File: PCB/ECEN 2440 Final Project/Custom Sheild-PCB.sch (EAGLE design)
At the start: 10 parts

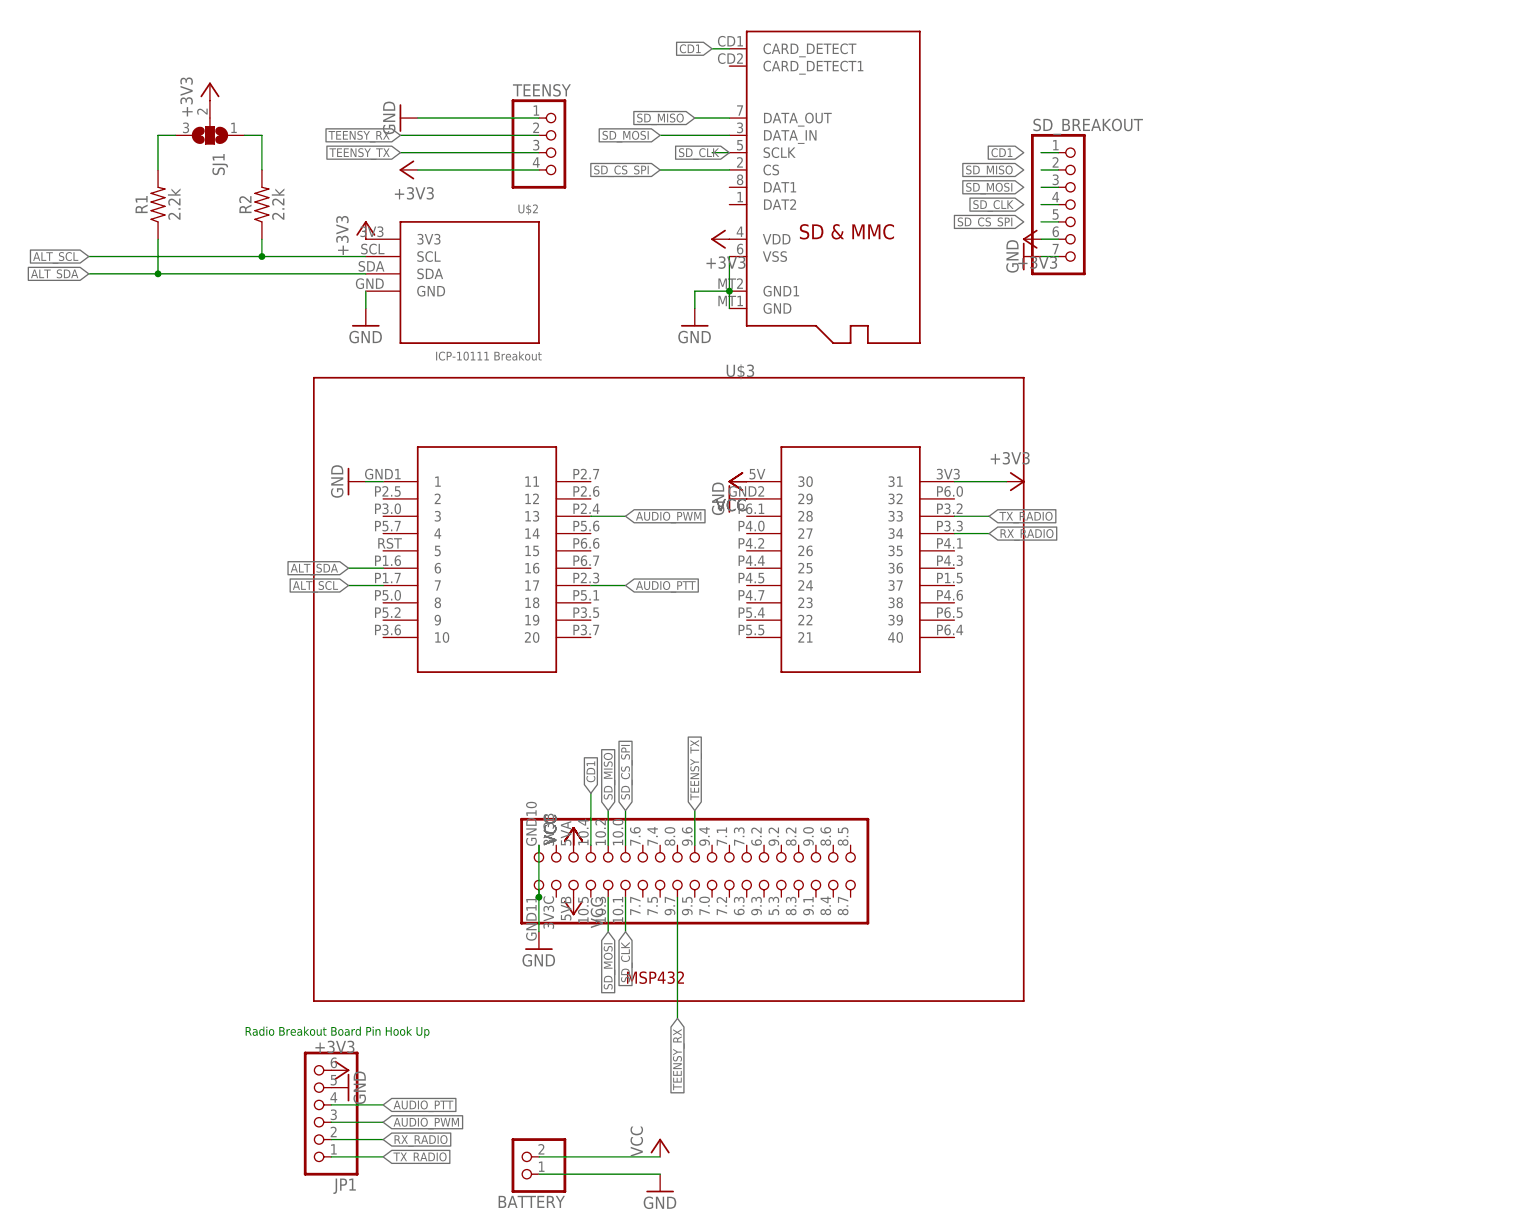
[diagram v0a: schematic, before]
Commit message: prettyfy schematic. vague shield board layout.
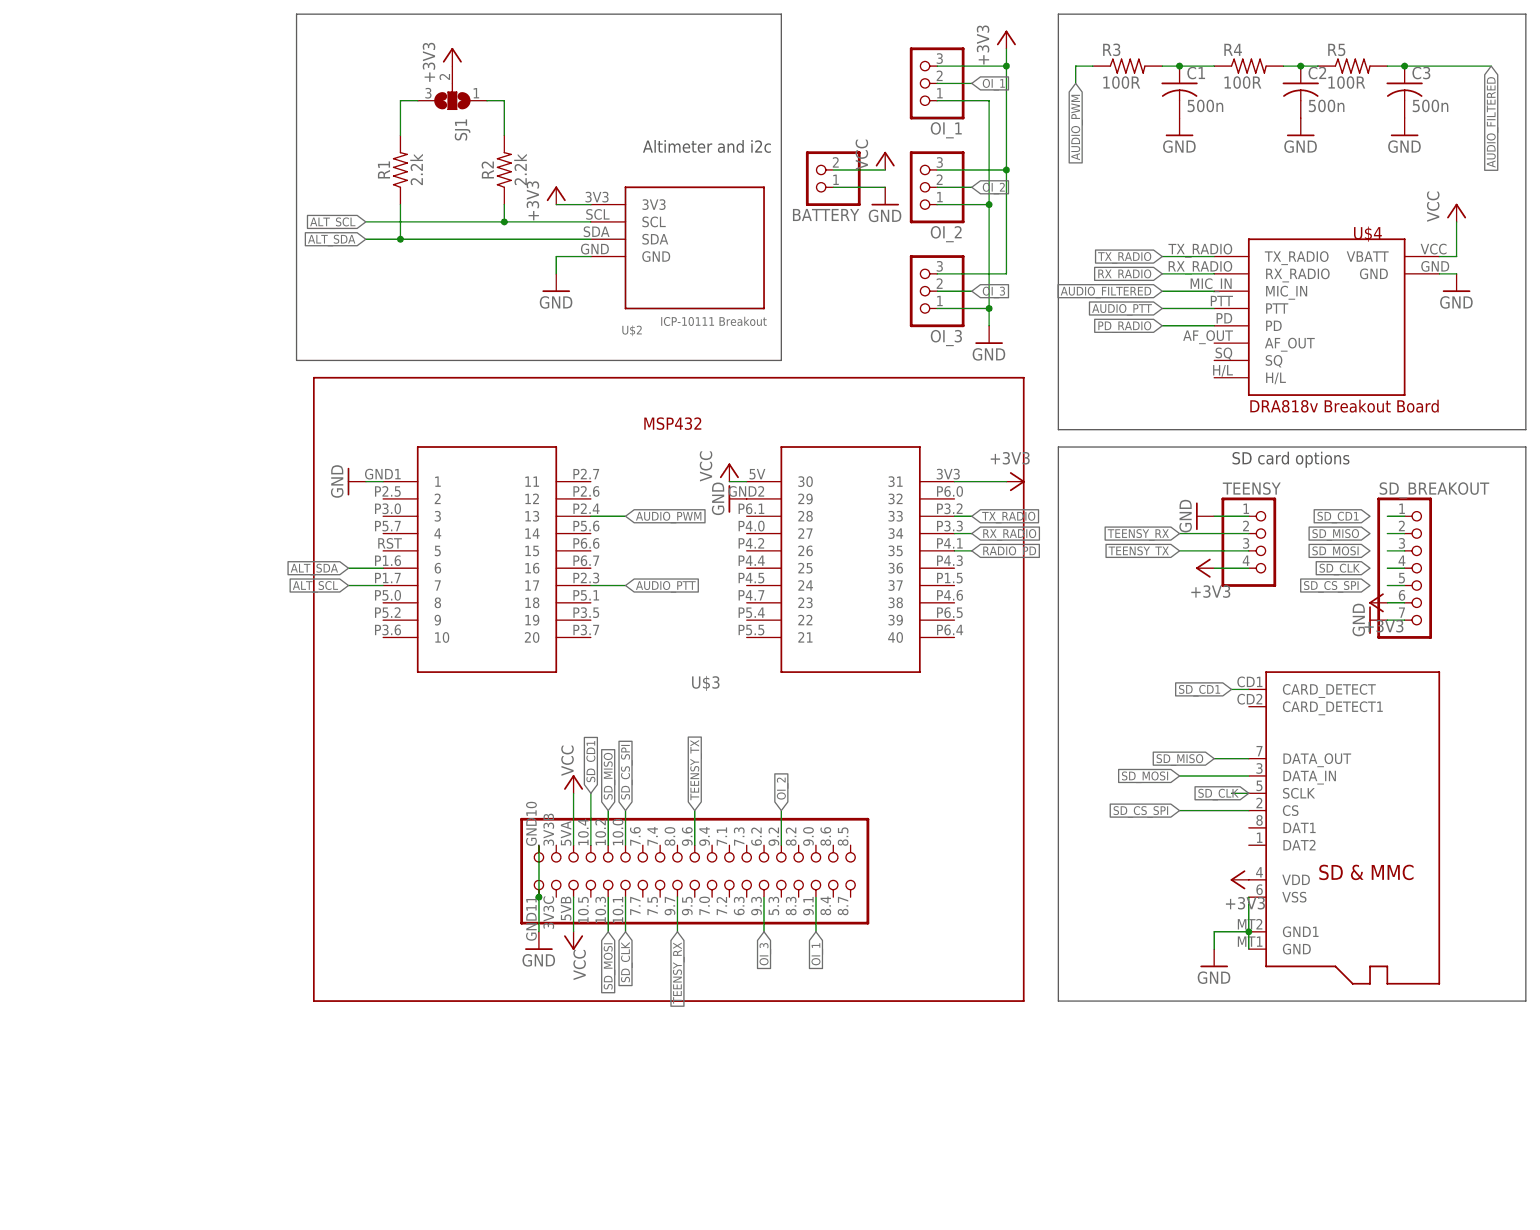
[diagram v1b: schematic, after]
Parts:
- removed JP1: (no value), pinhead:PINHD-1X6
- added C1, C2, C3: 500n, rcl:C-USC0805
- added OI_1, OI_2, OI_3: (no value), pinhead:PINHD-1X3
- added R3, R4, R5: 100R, rcl:R-US_R0805
- added U$4: DRA_BREAKOUT, Custom Library:DRA_BREAKOUT
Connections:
- net CD1 renamed SD_CD1
- new net AUDIO_FILTERED: C3.1, R5.2, U$4.MIC_IN
- new net N$3: C1.1, R3.2, R4.1
- new net N$4: C2.1, R4.2, R5.1
- new net OI_1: OI_1.2, U$3.73
- new net OI_2: OI_2.2, U$3.70
- new net OI_3: OI_3.2, U$3.67
- new net PD_RADIO: U$4.PD
- new net RADIO_PD: U$3.35
- net +3V3: now also OI_1.3, OI_2.3, OI_3.3; no longer JP1.6
- net AUDIO_PTT: now also U$4.PTT; no longer JP1.4
- net AUDIO_PWM: now also R3.1; no longer JP1.3
- net GND: now also C1.2, C2.2, C3.2, OI_1.1, OI_2.1, OI_3.1, U$4.GND; no longer JP1.5
- net RX_RADIO: now also U$4.RX_RADIO; no longer JP1.2
- net TX_RADIO: now also U$4.TX_RADIO; no longer JP1.1
- net VCC: now also U$4.VBATT
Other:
- note added: "Altimeter and i2c"
- note added: "SD card options"
- note removed: "Radio Breakout Board Pin Hook Up"
- moved on the sheet: BATTERY, R1, R2, SD_BREAKOUT, SJ1, TEENSY, U$2
